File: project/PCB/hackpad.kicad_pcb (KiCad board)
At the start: 2 copper layers, 47.6 x 89.2 mm, 8 parts, among them SW1 SW_Push, SW2 SW_Push, SW3 SW_Push, SW4 SW_Push, SW5 SW_Push, U1 XIAO-RP2040-DIP

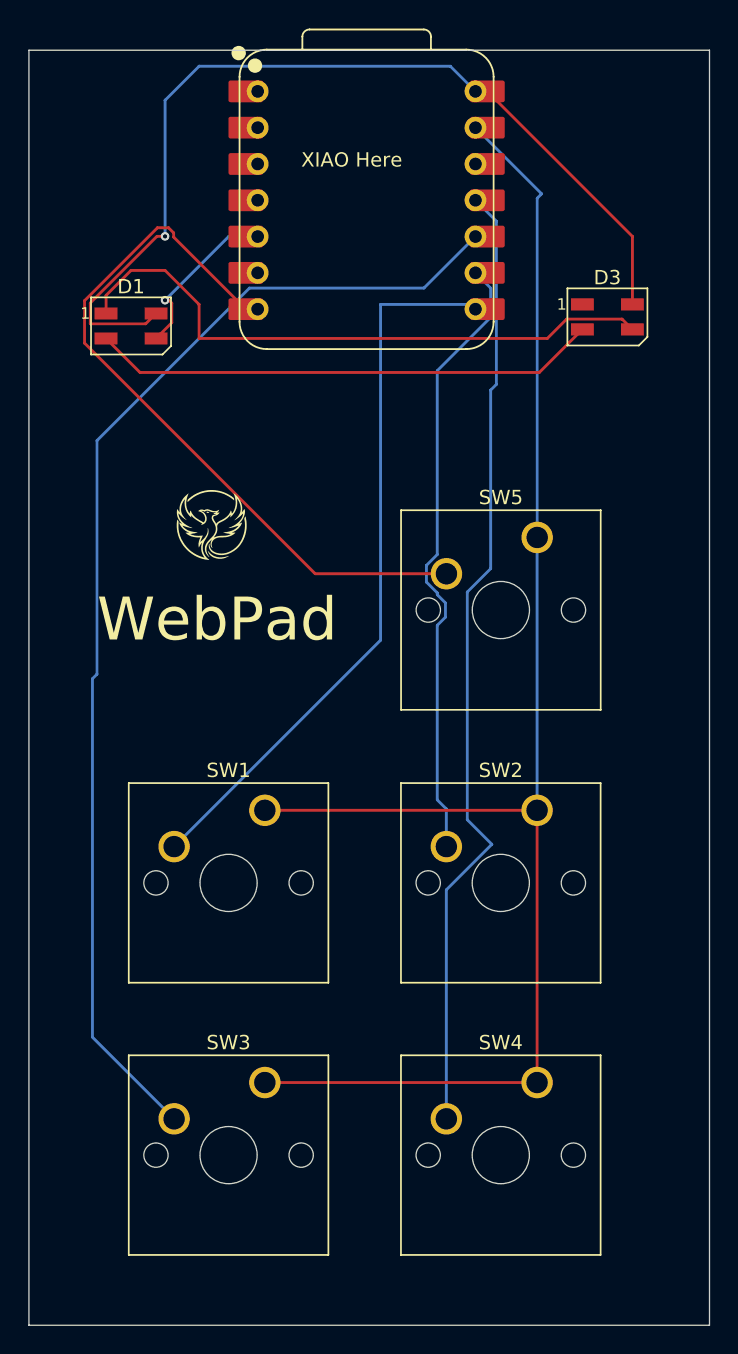
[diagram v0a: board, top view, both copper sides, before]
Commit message: Modify Readme Info and images
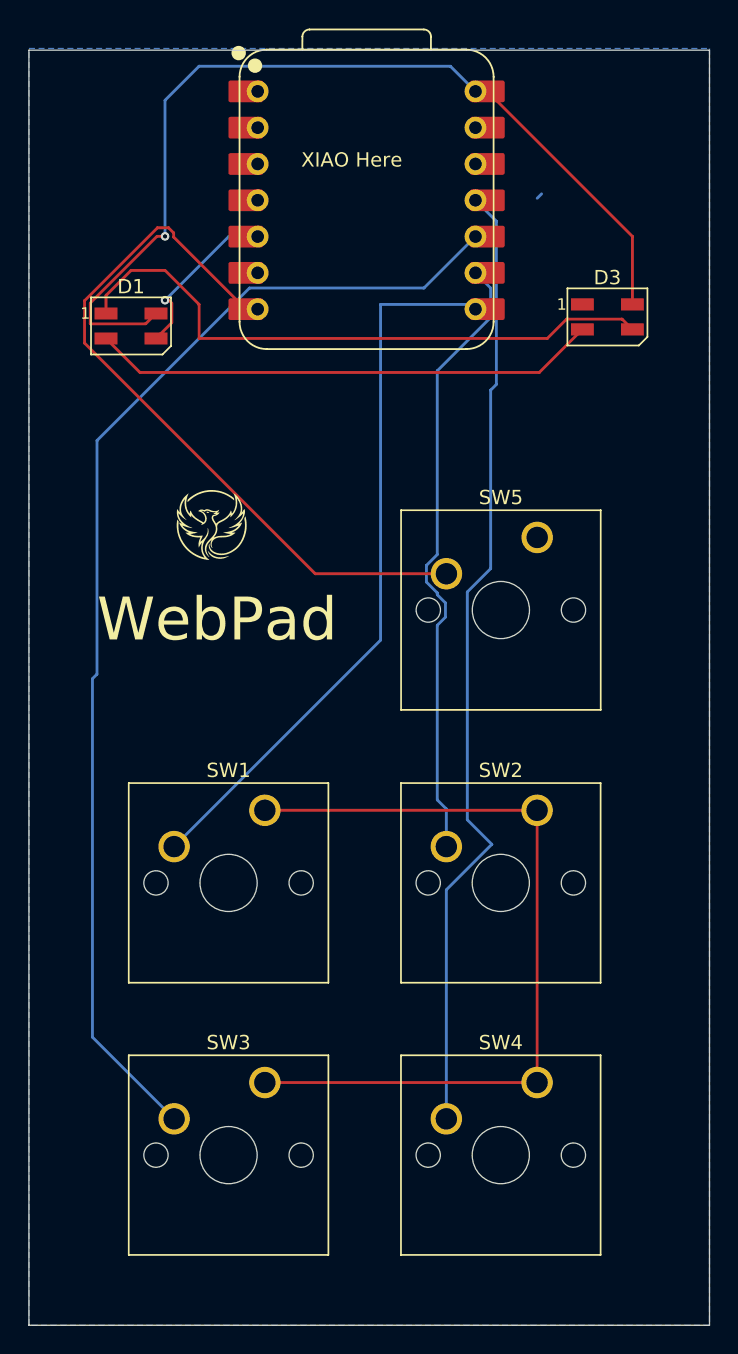
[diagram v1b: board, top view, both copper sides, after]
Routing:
- net GND: track 107.2 -> 57.6 mm
- added copper zone on B.Cu, net GND
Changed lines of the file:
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@@
 			(outputformat 1)
 			(mirror no)
-			(drillshape 1)
+			(drillshape 0)
 			(scaleselection 1)
 			(outputdirectory "")
@@
 	)
 	(segment
-		(start 202.2475 80.645)
-		(end 202.2475 61.317729)
-		(width 0.2)
-		(layer "B.Cu")
-		(net 6)
-	)
-	(segment
-		(start 202.565 37.505229)
-		(end 197.934992 32.875221)
-		(width 0.2)
-		(layer "B.Cu")
-		(net 6)
-	)
-	(segment
 		(start 202.565 37.505229)
 		(end 202.253757 37.816472)
@@
 	)
 	(segment
-		(start 202.253757 37.816472)
-		(end 202.253757 61.550724)
-		(width 0.2)
-		(layer "B.Cu")
-		(net 6)
-	)
-	(segment
 		(start 176.8475 83.185)
 		(end 191.29375 68.73875)
@@
 		(net 14)
 	)
+	(zone
+		(net 6)
+		(net_name "GND")
+		(layer "B.Cu")
+		(hatch edge 0.5)
+		(connect_pads
+			(clearance 0.5)
+		)
+		(min_thickness 0.25)
+		(filled_areas_thickness no)
+		(fill yes
+			(thermal_gap 0.5)
+			(thermal_bridge_width 0.5)
+		)
+		(polygon
+			(pts
+				(xy 166.6875 27.336155) (xy 214.3125 27.336155) (xy 214.3125 116.68125) (xy 166.6875 116.68125)
+			)
+		)
+	)
 	(group ""
